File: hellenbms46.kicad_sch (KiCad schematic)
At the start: 0 parts

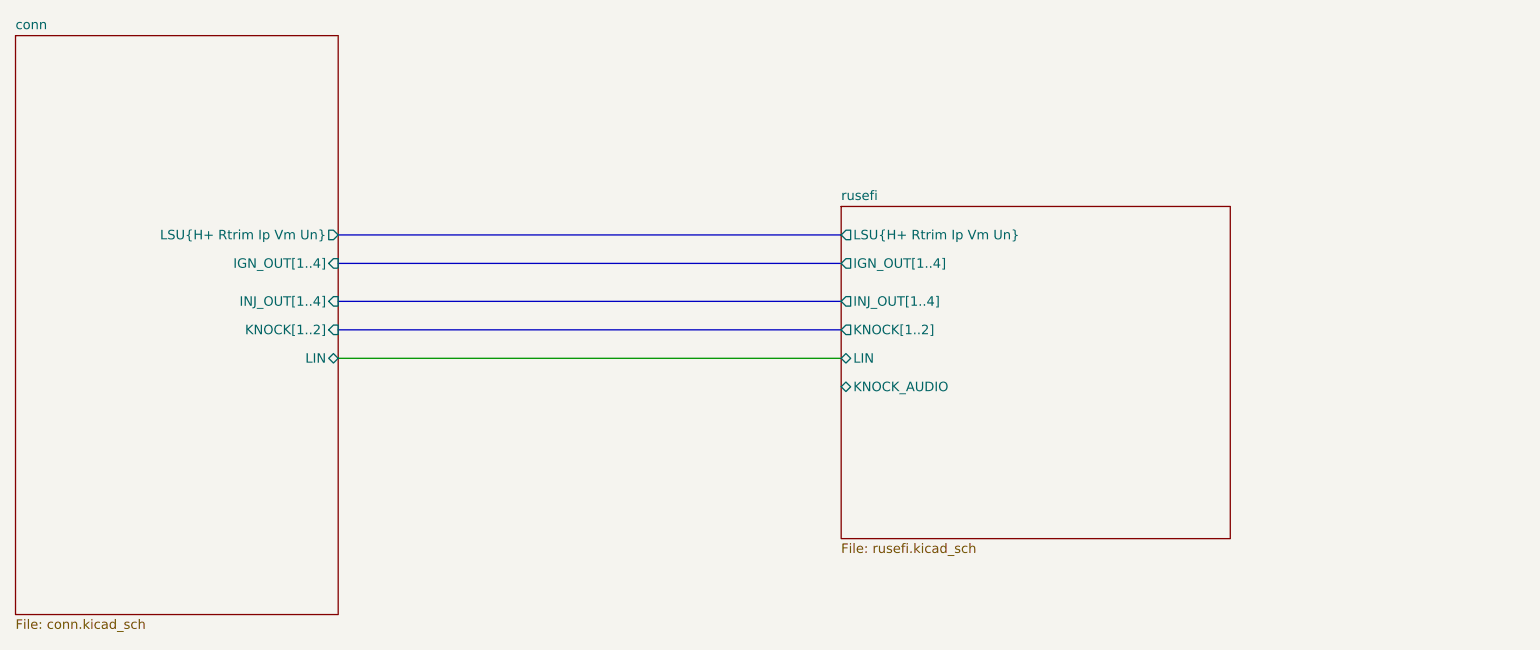
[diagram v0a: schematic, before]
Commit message: Initial schematic
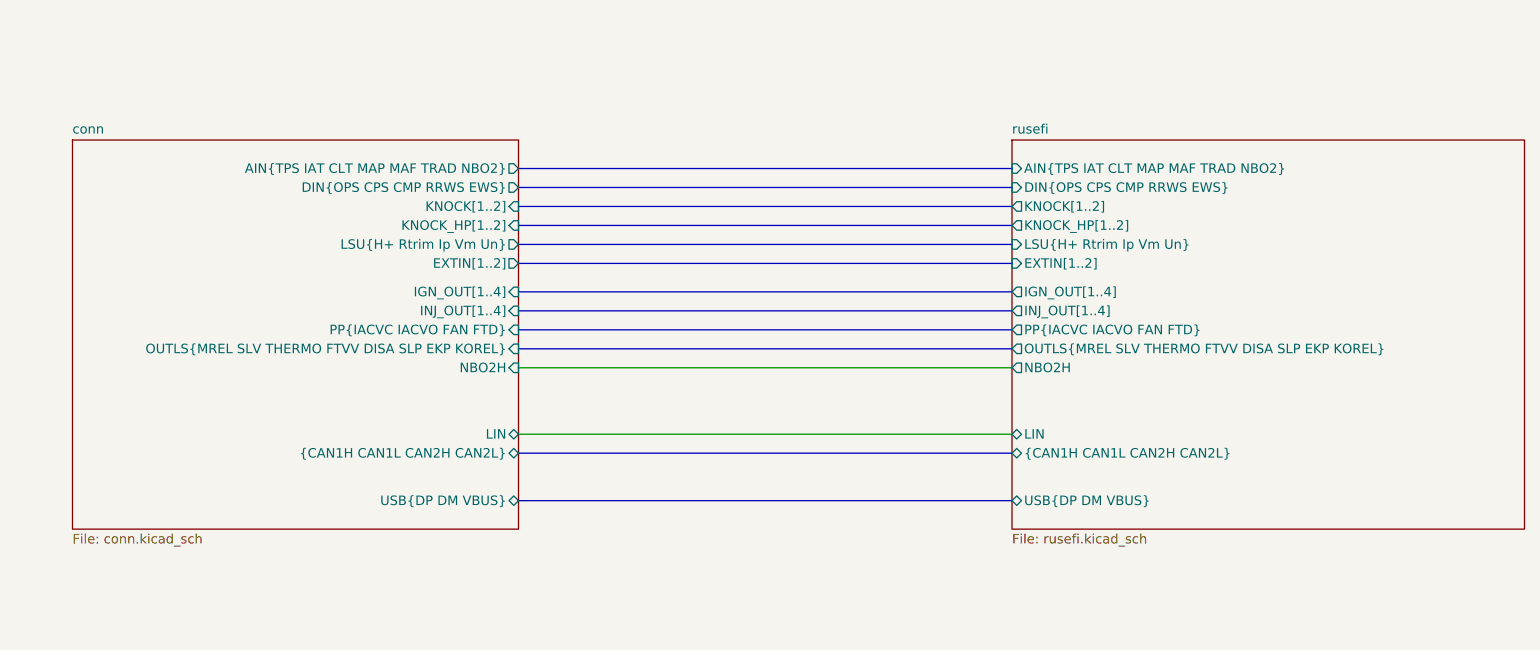
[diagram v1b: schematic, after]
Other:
- sheet conn ports: added AIN{TPS IAT CLT MAP MAF TRAD NBO2}, DIN{OPS CPS CMP RRWS EWS}, EXTIN[1..2], KNOCK_HP[1..2], NBO2H, OUTLS{MREL SLV THERMO FTVV DISA SLP EKP KOREL}, PP{IACVC IACVO FAN FTD}, USB{DP DM VBUS}, {CAN1H CAN1L CAN2H CAN2L}; removed none
- sheet rusefi ports: added AIN{TPS IAT CLT MAP MAF TRAD NBO2}, DIN{OPS CPS CMP RRWS EWS}, EXTIN[1..2], KNOCK_HP[1..2], NBO2H, OUTLS{MREL SLV THERMO FTVV DISA SLP EKP KOREL}, PP{IACVC IACVO FAN FTD}, USB{DP DM VBUS}, {CAN1H CAN1L CAN2H CAN2L}; removed KNOCK_AUDIO
